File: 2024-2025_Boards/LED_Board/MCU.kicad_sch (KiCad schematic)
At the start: 13 parts, among them J2 Conn_01x02_Pin, J3 Conn_01x02_Pin, J4 Conn_ARM_JTAG_SWD_10, U3 STM32G431CBT6

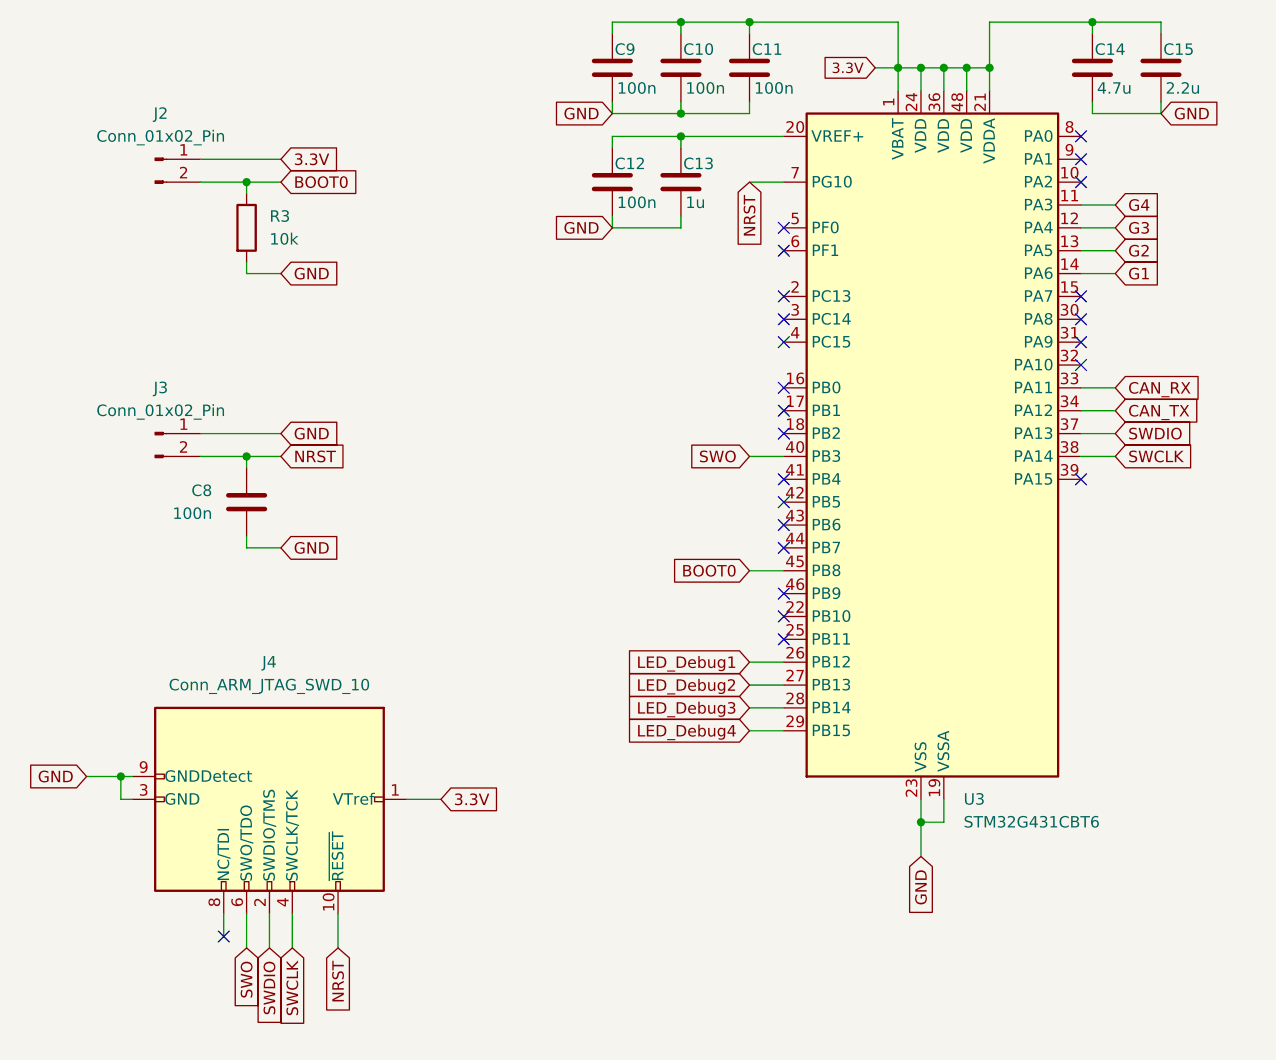
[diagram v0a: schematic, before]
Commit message: Pins on correct side
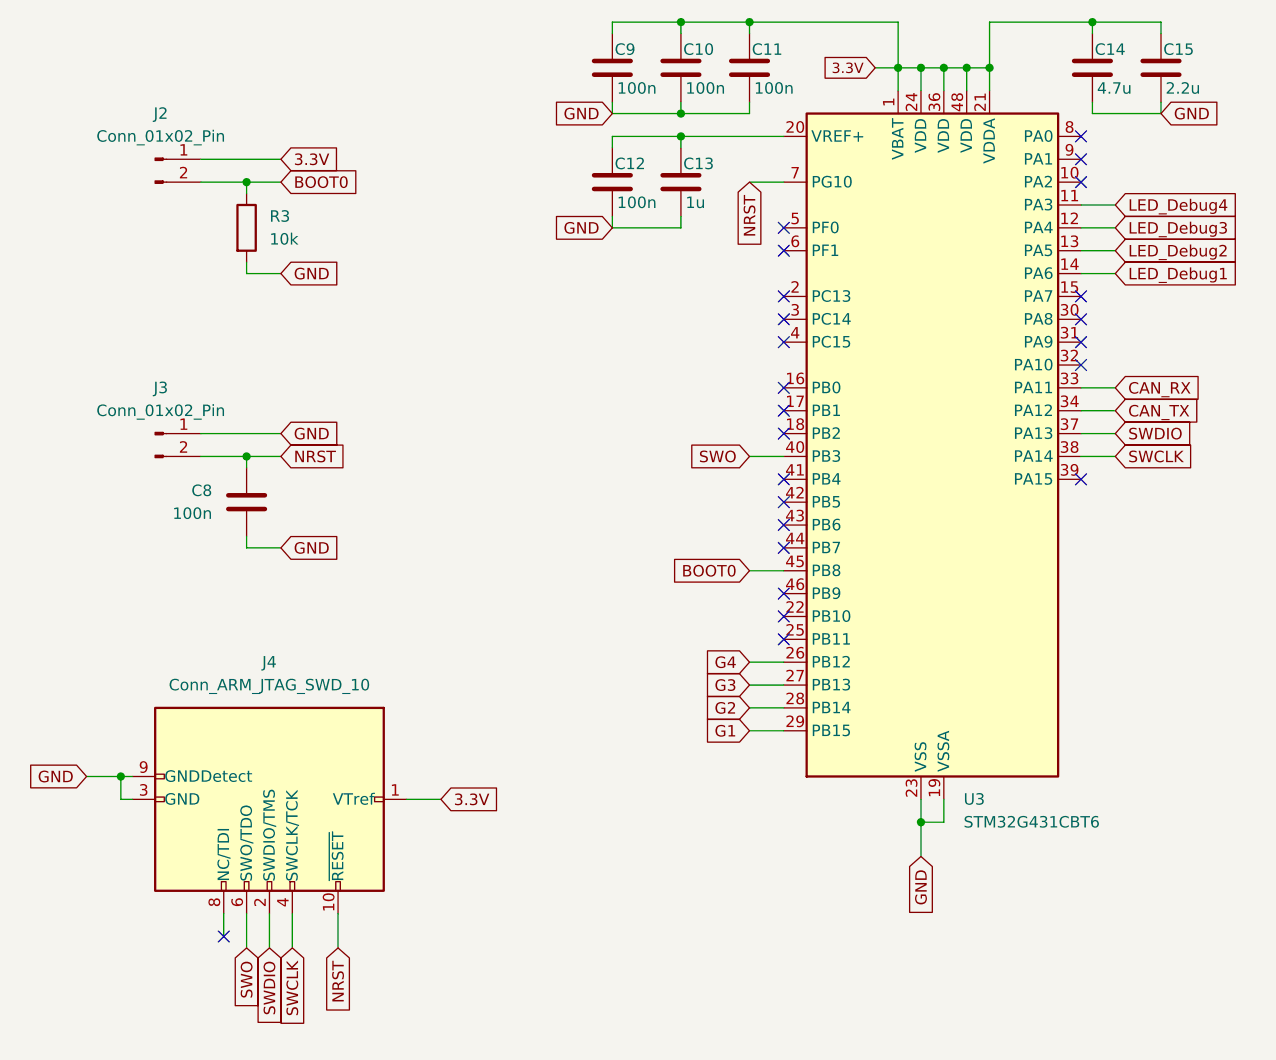
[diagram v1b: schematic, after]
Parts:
- J2, J3: footprint Cornell_Mars_Rover:CONN_PH1RB-02-UA_ADM -> Connector_PinHeader_2.54mm:PinHeader_1x02_P2.54mm_Horizontal
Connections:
- net G1: now also U3.29 (PB15); no longer U3.14 (PA6)
- net G2: now also U3.28 (PB14); no longer U3.13 (PA5)
- net G3: now also U3.27 (PB13); no longer U3.12 (PA4)
- net G4: now also U3.26 (PB12); no longer U3.11 (PA3)
- net LED_Debug1: now also U3.14 (PA6); no longer U3.26 (PB12)
- net LED_Debug2: now also U3.13 (PA5); no longer U3.27 (PB13)
- net LED_Debug3: now also U3.12 (PA4); no longer U3.28 (PB14)
- net LED_Debug4: now also U3.11 (PA3); no longer U3.29 (PB15)

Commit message: Board fixes
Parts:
- C14, C15: footprint Capacitor_SMD:C_0402_1005Metric -> Capacitor_SMD:C_0603_1608Metric
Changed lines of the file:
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@@
 			)
 		)
-		(property "Footprint" "Capacitor_SMD:C_0402_1005Metric"
+		(property "Footprint" "Capacitor_SMD:C_0603_1608Metric"
 			(at 172.4152 49.53 0)
 			(effects
@@
 			)
 		)
-		(property "Footprint" "Capacitor_SMD:C_0402_1005Metric"
+		(property "Footprint" "Capacitor_SMD:C_0603_1608Metric"
 			(at 180.0352 49.53 0)
 			(effects
